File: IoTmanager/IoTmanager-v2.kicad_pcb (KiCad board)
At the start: 2 copper layers, 48 x 75 mm, 62 parts, among them J2 Conn_01x12_Pin, J3 Conn_01x12_Pin, J4-flash1 flash, J5 reset, K3 ZC32F-012-HS3-copy, K5 ZC32F-012-HS3-copy, K6 ZC32F-012-HS3-copy, K7 ZC32F-012-HS3-copy, SW1 SW_PUSH_6mm_H4.3mm, U10 MMDT4413-7-F, U11 MMDT4413-7-F, U12 AMS1117-5.0, U2 ESP-12F, U3 DHT11, U3-tsop23 TSOP23xx, U5 PJ-320A, U6 AMS1117-3.3, U7 DS18B20, U8 MMDT4413-7-F, U9 MMDT4413-7-F

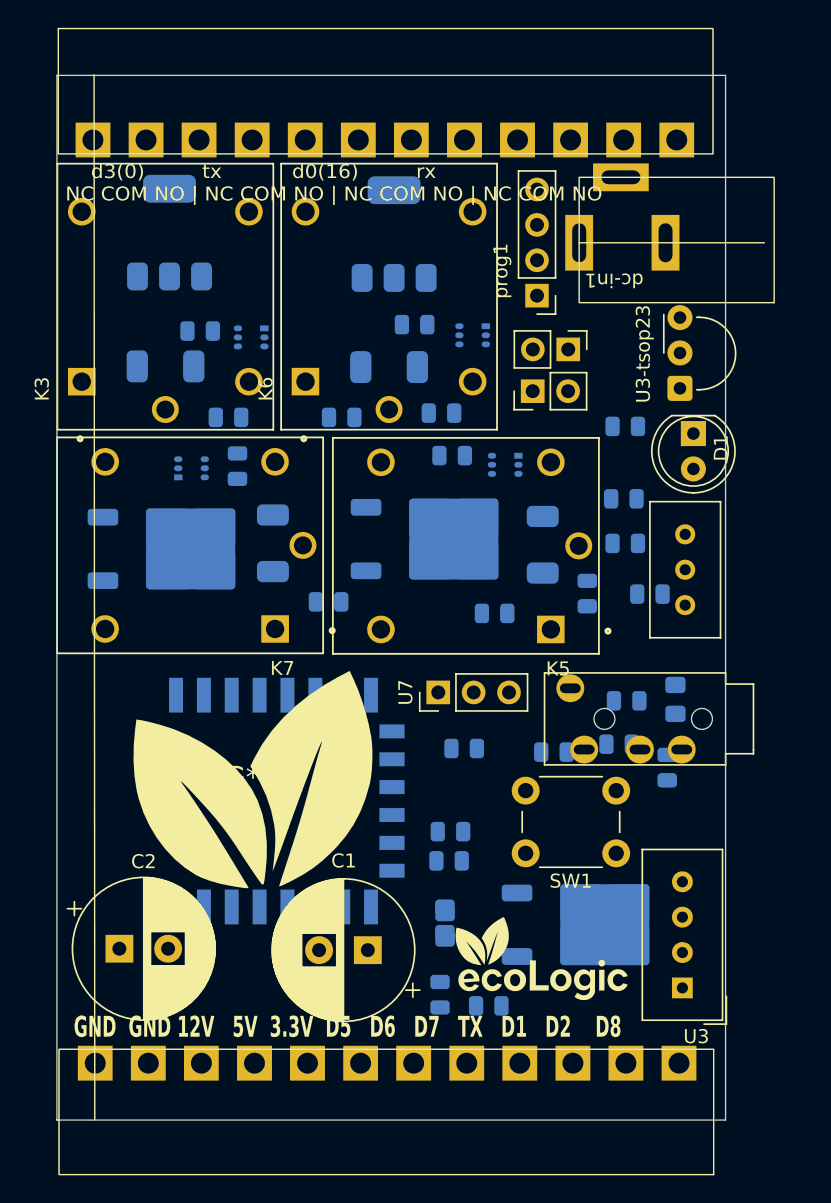
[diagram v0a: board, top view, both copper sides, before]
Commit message: update
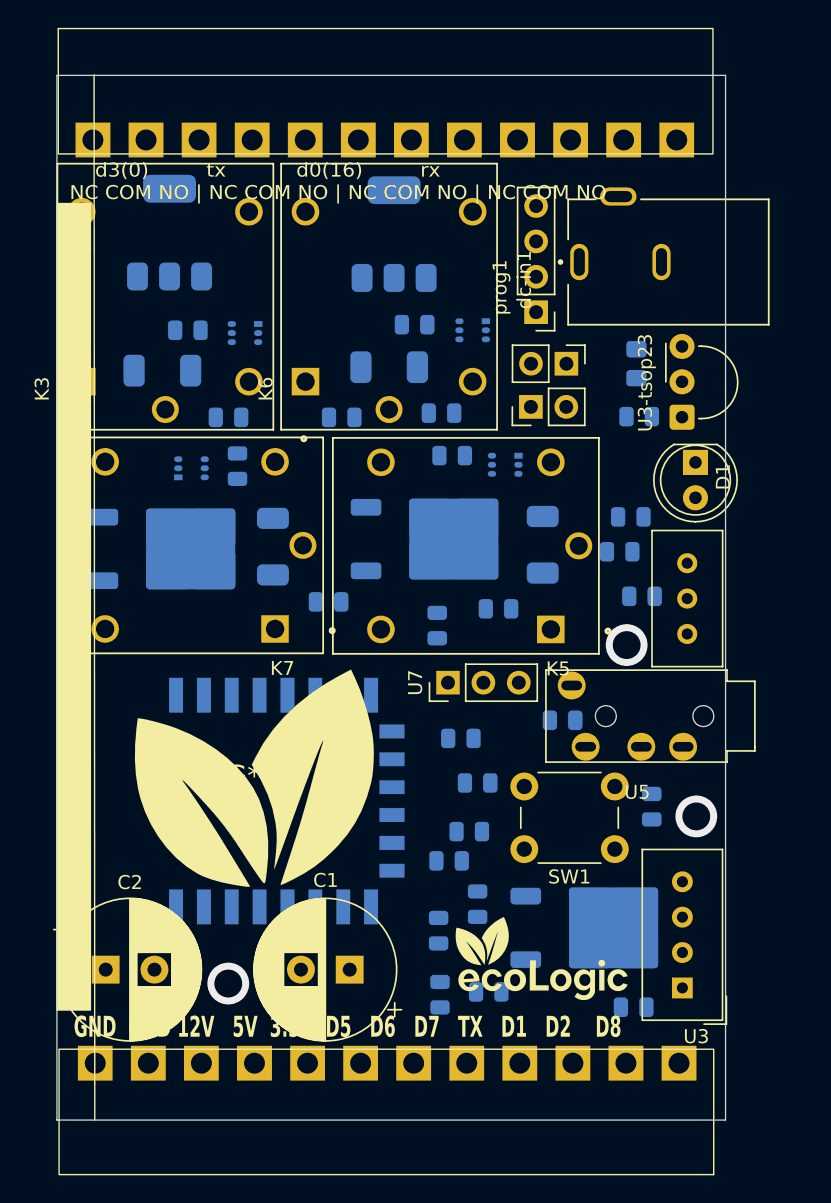
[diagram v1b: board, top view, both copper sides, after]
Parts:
- dc-in1: footprint module-custom-for-esp8266:dc-in-plastic-standard -> module-custom-for-esp8266:5.5PowerIn
- moved R12-10k4 36.5 mm to (119.0, 121.8)
- moved C3 24.3 mm to (119.2, 75.6), turned to -90 degrees
- moved R16 13.2 mm to (118.8, 86.6)
- moved R1 11.0 mm to (104.9, 94.4)
- moved dc-in1 6.07 mm to (121.0, 68.3), turned to 90 degrees
- moved R12-10k2 5.92 mm to (107.8, 105.7)
- moved R13 4.41 mm to (113.9, 101.2)
- moved R7 3.02 mm to (120.3, 107.4)
- moved R6 2.59 mm to (107.8, 114.4), turned to 90 degrees
- moved D1 2.08 mm to (123.4, 82.7)
- moved RV1 2.08 mm to (122.8, 89.9)
- moved U3-tsop23 2.08 mm to (122.5, 79.4)
- moved C1 1.91 mm to (98.6, 119.1)
- moved C2 1.79 mm to (81.1, 119.1)
- moved Jumper-d6 1.35 mm to (107.2, 109.2)
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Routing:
- net /a0: vias 0 -> 1
- net (no net): vias 0 -> 2

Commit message: update
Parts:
- U8: value MMDT4413-7-F -> MMDT4413
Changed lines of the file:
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@@
 			)
 			(scale
-				(xyz 1 1 1)
+				(xyz 1 1 1.7)
 			)
 			(rotate
@@
 			)
 			(scale
-				(xyz 1 1 1)
+				(xyz 1 1 1.7)
 			)
 			(rotate
@@
 		(at 127.705 103.1 180)
 		(property "Reference" "U5"
-			(at 8.4455 -3.269 360)
+			(at 8.4455 -3.269 0)
 			(layer "F.SilkS")
 			(effects
@@
 		)
 		(property "Value" "PJ-320A"
-			(at 8.4455 -4.539 360)
+			(at 8.4455 -4.539 0)
 			(layer "F.Fab")
 			(effects
@@
 		)
 		(property "Footprint" "module-custom-for-esp8266:PJ-320A"
-			(at 0 0 360)
+			(at 0 0 0)
 			(layer "F.Fab")
 			(hide yes)
@@
 		)
 		(property "Datasheet" ""
-			(at 0 0 360)
+			(at 0 0 0)
 			(layer "F.Fab")
 			(hide yes)
@@
 		)
 		(property "Description" ""
-			(at 0 0 360)
+			(at 0 0 0)
 			(layer "F.Fab")
 			(hide yes)
@@
 		(tags "resistor")
 		(property "Reference" "Jumper-d5"
-			(at -1.85 0.26 360)
+			(at -1.85 0.26 0)
 			(layer "B.SilkS")
 			(hide yes)
@@
 		)
 		(property "Value" "1"
-			(at 2.5125 -0.6 360)
+			(at 2.5125 -0.6 0)
 			(layer "B.Fab")
 			(effects
@@
 		)
 		(fp_text user "${REFERENCE}"
-			(at 1.0125 0.3 360)
+			(at 1.0125 0.3 0)
 			(layer "B.Fab")
 			(effects
@@
 			)
 		)
-		(property "Value" "MMDT4413-7-F"
+		(property "Value" "MMDT4413"
 			(at -0.3 2.2 0)
 			(unlocked yes)
